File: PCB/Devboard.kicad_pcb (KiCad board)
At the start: 2 copper layers, 675 parts, among them CN1 APCI0120-P001A, J1 HR911105A_C12074, J10 I2C_7, J11 3.3V_I2C, J17 I2C_0, J2 USB3_B, J4 I2C_1, J5 I2C_2, J6 I2C_3, J7 I2C_4, J8 I2C_5, J9 I2C_6, Q1 IPB180P04P4L-02, Q2 IPB180P04P4L-02, SW1 SW_Push, U1 TVS2201DRBR, U10 TPS62822DLCR, U11 TPS62823DLCR, U12 TPS548A20RVER, U13 TPS7A4700RGWR, U14 TPS3700DSET, U15 TPS54824RNVR, U16 TPS54824RNVR, U17 TPS7A4700RGWR, U18 DW06, U19 TPS61088RHLR, U2 TPD6S300ARUKR, U20 TPS54824RNVR, U21 LM66100DCK, U22 TPS7A4700RGWR, U23 TPS7A4700RGWR, U24 TPS259470ARPWR, U25 TPS54824RNVR, U26 xczu4evfbvb900pkg, U27 RS3112-1.25XSF3, U28 MT25QU256ABA8ESF-0SIT TR, U29 FEMDNN032G-A3A55, U3 STUSB4500QTR, U30 TXS02612RTWR, U31 DP83867IRRGZR, U32 USB3320C-EZK-TR, U33 TPD4E05U06DQA, U34 CP2102N-A02-GQFN24, U35 TXB0108PW, U36 TCA9548APWR, U37 PCA9306, U39 TPD4E05U06DQA, U4 TPS2121RUXR, U40 USB2514B_Bi, U5 TPS259470ARPWR, U6 BQ25895RTWR, U7 BQ27441DRZR-G1A, U8 TPS62130RGTR, U9 XT60, Y1 25 MHz, Y2 25 MHz, Y4 26 MHz

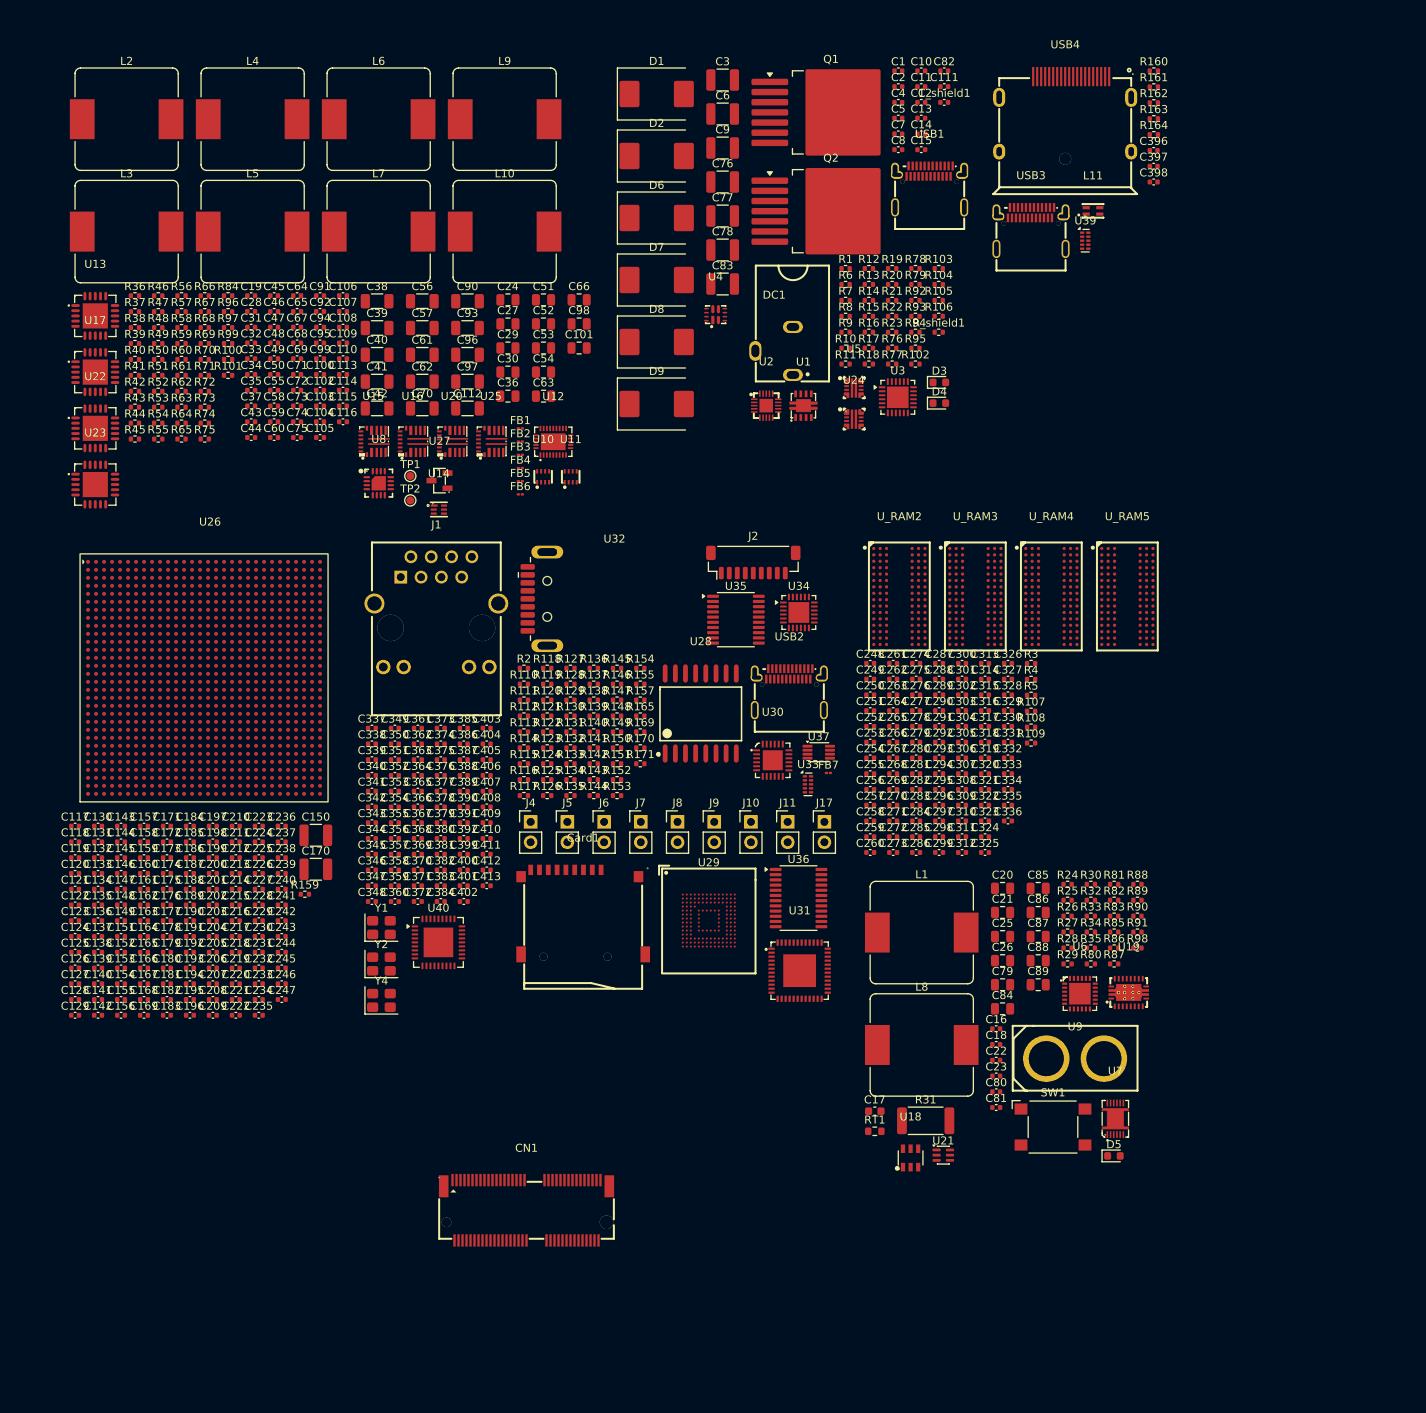
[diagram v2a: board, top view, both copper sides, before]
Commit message: Feat : Schematics Complete
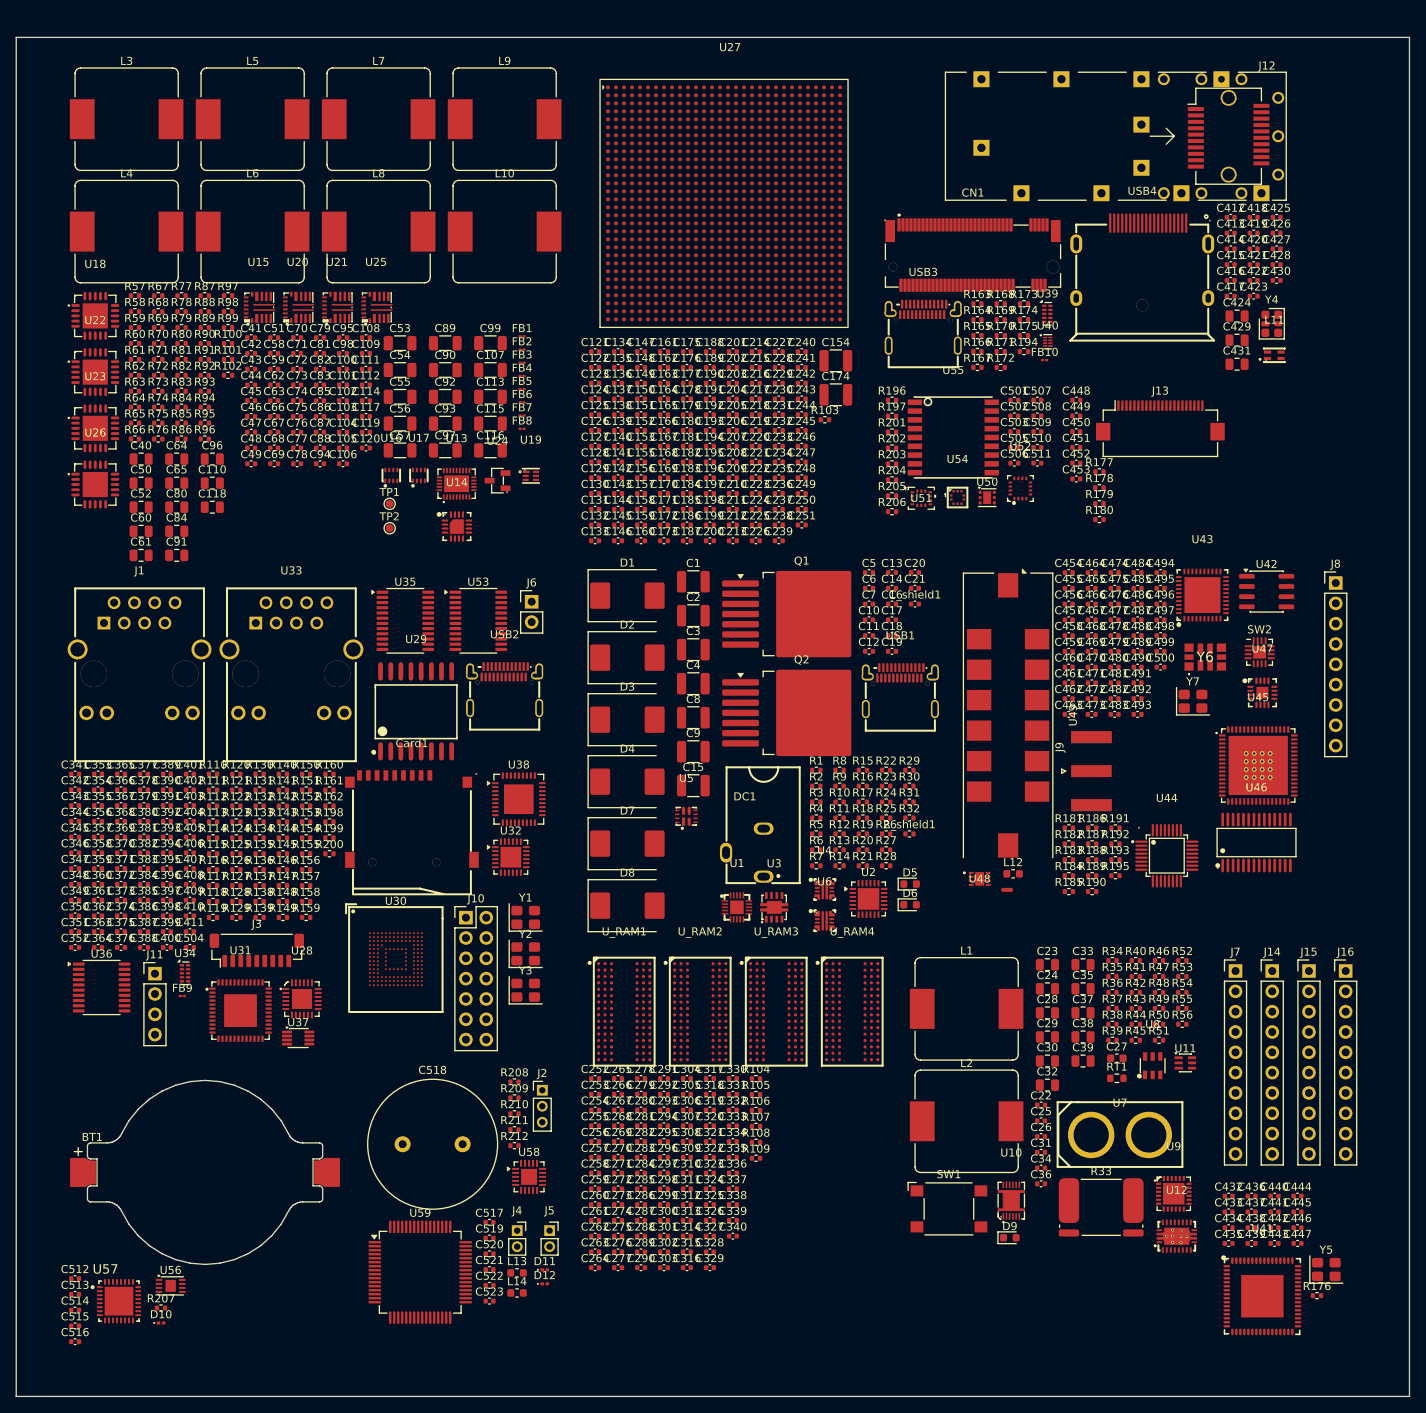
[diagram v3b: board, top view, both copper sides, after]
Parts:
- removed J17: I2C_0, Connector_PinHeader_2.54mm:PinHeader_1x02_P2.54mm_Vertical
- removed U_RAM5: MT40A512M16LY-075:E, Devboard_Footprints:FBGA-96_L13.5-W7.5-R16-C6-P0.80-TL
- added BT1: Battery_Cell, Battery:BatteryHolder_Keystone_1057_1x2032, F.Cu at (17.2, 138.2)
- added C393: 1uF, Capacitor_SMD:C_0402_1005Metric, F.Cu at (12.4, 96.3)
- added C394: 1uF, Capacitor_SMD:C_0402_1005Metric, F.Cu at (12.4, 98.2)
- added C395: 1uF, Capacitor_SMD:C_0402_1005Metric, F.Cu at (12.4, 100.2)
- added C414: 100nF, Capacitor_SMD:C_0402_1005Metric, F.Cu at (145.4, 22.7)
- added C415: 100nF, Capacitor_SMD:C_0402_1005Metric, F.Cu at (145.4, 24.7)
- added C416: 100nF, Capacitor_SMD:C_0402_1005Metric, F.Cu at (145.4, 26.7)
- added C417: 100nF, Capacitor_SMD:C_0402_1005Metric, F.Cu at (145.4, 28.6)
- added C418: 100nF, Capacitor_SMD:C_0402_1005Metric, F.Cu at (148.3, 18.8)
- added C419: 100nF, Capacitor_SMD:C_0402_1005Metric, F.Cu at (148.3, 20.8)
- added C420: 100nF, Capacitor_SMD:C_0402_1005Metric, F.Cu at (148.3, 22.7)
- added C421: 100nF, Capacitor_SMD:C_0402_1005Metric, F.Cu at (148.3, 24.7)
- added C422: 1nF, Capacitor_SMD:C_0402_1005Metric, F.Cu at (148.3, 26.7)
- added C423: 100nF, Capacitor_SMD:C_0402_1005Metric, F.Cu at (148.3, 28.6)
- added C424: 10uF, Capacitor_SMD:C_0805_2012Metric, F.Cu at (146.2, 31.1)
- added C425: 100nF, Capacitor_SMD:C_0402_1005Metric, F.Cu at (151.1, 18.8)
- added C426: 100nF, Capacitor_SMD:C_0402_1005Metric, F.Cu at (151.1, 20.8)
- added C427: 100nF, Capacitor_SMD:C_0402_1005Metric, F.Cu at (151.1, 22.7)
- added C428: 100nF, Capacitor_SMD:C_0402_1005Metric, F.Cu at (151.1, 24.7)
- added C429: 10uF, Capacitor_SMD:C_0805_2012Metric, F.Cu at (146.2, 34.1)
- added C430: 100nF, Capacitor_SMD:C_0402_1005Metric, F.Cu at (151.1, 26.7)
- added C431: 10uF, Capacitor_SMD:C_0805_2012Metric, F.Cu at (146.2, 37.2)
- added C432: 0.1uF, Capacitor_SMD:C_0402_1005Metric, F.Cu at (145.1, 141.1)
- added C433: 0.1uF, Capacitor_SMD:C_0402_1005Metric, F.Cu at (145.1, 143.1)
- added C434: 0.1uF, Capacitor_SMD:C_0402_1005Metric, F.Cu at (145.1, 145.1)
- added C435: 0.1uF, Capacitor_SMD:C_0402_1005Metric, F.Cu at (145.1, 147.1)
- added C436: 0.1uF, Capacitor_SMD:C_0402_1005Metric, F.Cu at (148.0, 141.1)
- added C437: 0.1uF, Capacitor_SMD:C_0402_1005Metric, F.Cu at (148.0, 143.1)
- added C438: 0.1uF, Capacitor_SMD:C_0402_1005Metric, F.Cu at (148.0, 145.1)
- added C439: 0.1uF, Capacitor_SMD:C_0402_1005Metric, F.Cu at (148.0, 147.1)
- added C440: 0.1uF, Capacitor_SMD:C_0402_1005Metric, F.Cu at (150.9, 141.1)
- added C441: 0.1uF, Capacitor_SMD:C_0402_1005Metric, F.Cu at (150.9, 143.1)
- added C442: 0.1uF, Capacitor_SMD:C_0402_1005Metric, F.Cu at (150.9, 145.1)
- added C443: 0.1uF, Capacitor_SMD:C_0402_1005Metric, F.Cu at (150.9, 147.1)
- added C444: 0.1uF, Capacitor_SMD:C_0402_1005Metric, F.Cu at (153.7, 141.1)
- added C445: 0.1uF, Capacitor_SMD:C_0402_1005Metric, F.Cu at (153.7, 143.1)
- added C446: 0.1uF, Capacitor_SMD:C_0402_1005Metric, F.Cu at (153.7, 145.1)
- added C447: 0.1uF, Capacitor_SMD:C_0402_1005Metric, F.Cu at (153.7, 147.1)
- added C448: 100nF, Capacitor_SMD:C_0402_1005Metric, F.Cu at (126.1, 41.6)
- added C449: 100nF, Capacitor_SMD:C_0402_1005Metric, F.Cu at (126.1, 43.6)
- added C450: 100nF, Capacitor_SMD:C_0402_1005Metric, F.Cu at (126.1, 45.6)
- added C451: 10uF, Capacitor_SMD:C_0402_1005Metric, F.Cu at (126.1, 47.6)
- added C452: 100nF, Capacitor_SMD:C_0402_1005Metric, F.Cu at (126.1, 49.5)
- added C453: 10uF, Capacitor_SMD:C_0402_1005Metric, F.Cu at (126.1, 51.5)
- added C454: 10uF, Capacitor_SMD:C_0402_1005Metric, F.Cu at (125.1, 63.2)
- added C455: 10uF, Capacitor_SMD:C_0402_1005Metric, F.Cu at (125.1, 65.2)
- added C456: 100nF, Capacitor_SMD:C_0402_1005Metric, F.Cu at (125.1, 67.1)
- added C457: 1uF, Capacitor_SMD:C_0402_1005Metric, F.Cu at (125.1, 69.1)
- added C458: 100nF, Capacitor_SMD:C_0402_1005Metric, F.Cu at (125.1, 71.1)
- added C459: 1uF, Capacitor_SMD:C_0402_1005Metric, F.Cu at (125.1, 73.0)
- added C460: 100nF, Capacitor_SMD:C_0402_1005Metric, F.Cu at (125.1, 75.0)
- added C461: 100nF, Capacitor_SMD:C_0402_1005Metric, F.Cu at (125.1, 77.0)
- added C462: 100nF, Capacitor_SMD:C_0402_1005Metric, F.Cu at (125.1, 79.0)
- added C463: 100nF, Capacitor_SMD:C_0402_1005Metric, F.Cu at (125.1, 80.9)
- added C464: 100nF, Capacitor_SMD:C_0402_1005Metric, F.Cu at (128.0, 63.2)
- added C465: 10uF, Capacitor_SMD:C_0402_1005Metric, F.Cu at (128.0, 65.2)
- added C466: 1uF, Capacitor_SMD:C_0402_1005Metric, F.Cu at (128.0, 67.1)
- added C467: 100nF, Capacitor_SMD:C_0402_1005Metric, F.Cu at (128.0, 69.1)
- added C468: 1uF, Capacitor_SMD:C_0402_1005Metric, F.Cu at (128.0, 71.1)
- added C469: 10uF, Capacitor_SMD:C_0402_1005Metric, F.Cu at (128.0, 73.0)
- added C470: 1uF, Capacitor_SMD:C_0402_1005Metric, F.Cu at (128.0, 75.0)
- added C471: 100nF, Capacitor_SMD:C_0402_1005Metric, F.Cu at (128.0, 77.0)
- added C472: 1uF, Capacitor_SMD:C_0402_1005Metric, F.Cu at (128.0, 79.0)
- added C473: 0.56 nF, Capacitor_SMD:C_0402_1005Metric, F.Cu at (128.0, 80.9)
- added C474: 330 nF, Capacitor_SMD:C_0402_1005Metric, F.Cu at (130.9, 63.2)
- added C475: 3.3 nF, Capacitor_SMD:C_0402_1005Metric, F.Cu at (130.9, 65.2)
- added C476: 100nF, Capacitor_SMD:C_0402_1005Metric, F.Cu at (130.9, 67.1)
- added C477: 100pF, Capacitor_SMD:C_0402_1005Metric, F.Cu at (130.9, 69.1)
- added C478: 100pF, Capacitor_SMD:C_0402_1005Metric, F.Cu at (130.9, 71.1)
- added C479: 1uF, Capacitor_SMD:C_0402_1005Metric, F.Cu at (130.9, 73.0)
- added C480: 100nF, Capacitor_SMD:C_0402_1005Metric, F.Cu at (130.9, 75.0)
- added C481: 22pF, Capacitor_SMD:C_0402_1005Metric, F.Cu at (130.9, 77.0)
- added C482: 22pF, Capacitor_SMD:C_0402_1005Metric, F.Cu at (130.9, 79.0)
- added C483: 0.1uF, Capacitor_SMD:C_0402_1005Metric, F.Cu at (130.9, 80.9)
- added C484: 10uF, Capacitor_SMD:C_0402_1005Metric, F.Cu at (133.7, 63.2)
- added C485: 0.1uF, Capacitor_SMD:C_0402_1005Metric, F.Cu at (133.7, 65.2)
- added C486: 10uF, Capacitor_SMD:C_0402_1005Metric, F.Cu at (133.7, 67.1)
- added C487: 0.1uF, Capacitor_SMD:C_0402_1005Metric, F.Cu at (133.7, 69.1)
- added C488: 10uF, Capacitor_SMD:C_0402_1005Metric, F.Cu at (133.7, 71.1)
- added C489: 0.1uF, Capacitor_SMD:C_0402_1005Metric, F.Cu at (133.7, 73.0)
- added C490: 10uF, Capacitor_SMD:C_0402_1005Metric, F.Cu at (133.7, 75.0)
- added C491: 100nF, Capacitor_SMD:C_0402_1005Metric, F.Cu at (133.7, 77.0)
- added C492: 100nF, Capacitor_SMD:C_0402_1005Metric, F.Cu at (133.7, 79.0)
- added C493: 0.1uF, Capacitor_SMD:C_0402_1005Metric, F.Cu at (133.7, 80.9)
- added C494: 0.1uF, Capacitor_SMD:C_0402_1005Metric, F.Cu at (136.6, 63.2)
- added C495: 100pF, Capacitor_SMD:C_0402_1005Metric, F.Cu at (136.6, 65.2)
- added C496: 100pF, Capacitor_SMD:C_0402_1005Metric, F.Cu at (136.6, 67.1)
- added C497: 1uF, Capacitor_SMD:C_0402_1005Metric, F.Cu at (136.6, 69.1)
- added C498: 1uF, Capacitor_SMD:C_0402_1005Metric, F.Cu at (136.6, 71.1)
- added C499: 0.1 uF, Capacitor_SMD:C_0402_1005Metric, F.Cu at (136.6, 73.0)
- added C500: 100nF, Capacitor_SMD:C_0402_1005Metric, F.Cu at (136.6, 75.0)
- added C501: 0.1uF, Capacitor_SMD:C_0402_1005Metric, F.Cu at (118.3, 41.6)
- added C502: 0.1uF, Capacitor_SMD:C_0402_1005Metric, F.Cu at (118.3, 43.6)
- added C503: 0.1uF, Capacitor_SMD:C_0402_1005Metric, F.Cu at (118.3, 45.6)
- added C504: 0.1uF, Capacitor_SMD:C_0402_1005Metric, F.Cu at (15.3, 110.1)
- added C505: 0.1uF, Capacitor_SMD:C_0402_1005Metric, F.Cu at (118.3, 47.6)
- added C506: 0.1uF, Capacitor_SMD:C_0402_1005Metric, F.Cu at (118.3, 49.5)
- added C507: 10uF, Capacitor_SMD:C_0402_1005Metric, F.Cu at (121.2, 41.6)
- added C508: 0.1uF, Capacitor_SMD:C_0402_1005Metric, F.Cu at (121.2, 43.6)
- added C509: 0.1uF, Capacitor_SMD:C_0402_1005Metric, F.Cu at (121.2, 45.6)
- added C510: 0.1uF, Capacitor_SMD:C_0402_1005Metric, F.Cu at (121.2, 47.6)
- added C511: 0.1uF, Capacitor_SMD:C_0402_1005Metric, F.Cu at (121.2, 49.5)
- added C512: 0.1uF, Capacitor_SMD:C_0402_1005Metric, F.Cu at (0.94, 151.5)
- added C513: 0.1uF, Capacitor_SMD:C_0402_1005Metric, F.Cu at (0.94, 153.4)
- added C514: 0.1uF, Capacitor_SMD:C_0402_1005Metric, F.Cu at (0.94, 155.4)
- added C515: 0.1uF, Capacitor_SMD:C_0402_1005Metric, F.Cu at (0.94, 157.4)
- added C516: 0.1uF, Capacitor_SMD:C_0402_1005Metric, F.Cu at (0.94, 159.3)
- added C517: 0.1uF, Capacitor_SMD:C_0402_1005Metric, F.Cu at (52.7, 144.4)
- added C518: 22F 5.5V, Capacitor_THT:C_Radial_D16.0mm_H31.5mm_P7.50mm, F.Cu at (41.9, 134.7)
- added C519: 0.1uF, Capacitor_SMD:C_0402_1005Metric, F.Cu at (52.7, 146.4)
- added C520: 0.1uF, Capacitor_SMD:C_0402_1005Metric, F.Cu at (52.7, 148.4)
- added C521: 0.1uF, Capacitor_SMD:C_0402_1005Metric, F.Cu at (52.7, 150.3)
- added C522: 0.1uF, Capacitor_SMD:C_0402_1005Metric, F.Cu at (52.7, 152.3)
- added C523: 0.1uF, Capacitor_SMD:C_0402_1005Metric, F.Cu at (52.7, 154.3)
- added D10: RB521S30, Diode_SMD:D_0201_0603Metric, F.Cu at (11.7, 157.0)
- added D11: RB521S30, Diode_SMD:D_0201_0603Metric, F.Cu at (59.6, 150.4)
- added D12: RB521S30, Diode_SMD:D_0201_0603Metric, F.Cu at (59.6, 152.1)
- added FB10: 120Ω@100MHz, Inductor_SMD:L_01005_0402Metric, F.Cu at (122.1, 36.6)
- added FB8: 120Ω@100MHz, Inductor_SMD:L_01005_0402Metric, F.Cu at (56.8, 45.2)
- added FB9: BLM18, Inductor_SMD:L_01005_0402Metric, F.Cu at (14.3, 116.1)
- added J12: SFP+, Connector:Connector_SFP_and_Cage, F.Cu at (151.3, 8.65)
- added J13: Conn_01x22, Connector_FFC-FPC:Hirose_FH12-22S-0.5SH_1x22-1MP_P0.50mm_Horizontal, F.Cu at (136.6, 44.2)
- added J14: Conn_01x10, Connector_PinHeader_2.54mm:PinHeader_1x10_P2.54mm_Vertical, F.Cu at (150.6, 113.0)
- added J15: Conn_01x10, Connector_PinHeader_2.54mm:PinHeader_1x10_P2.54mm_Vertical, F.Cu at (155.2, 113.0)
- added J16: Conn_01x10, Connector_PinHeader_2.54mm:PinHeader_1x10_P2.54mm_Vertical, F.Cu at (159.8, 113.0)
- added J3: USB3_B, Connector_JST:JST_SH_BM09B-SRSS-TB_1x09-1MP_P1.00mm_Vertical, F.Cu at (23.6, 110.4)
- added L12: 220 nH, Inductor_SMD:L_0603_1608Metric, F.Cu at (118.2, 100.9)
- added L13: 220 nH, Inductor_SMD:L_0603_1608Metric, F.Cu at (56.2, 150.7)
- added L14: 220 nH, Inductor_SMD:L_0603_1608Metric, F.Cu at (56.2, 153.2)
- added NT1: NetTie_2, NetTie:NetTie-2_SMD_Pad0.5mm, F.Cu at (117.4, 102.9)
- added R156: 2.2kΩ, Resistor_SMD:R_0402_1005Metric, F.Cu at (29.8, 100.3)
- added R158: 10kΩ, Resistor_SMD:R_0402_1005Metric, F.Cu at (29.8, 104.3)
- added R166: 100kΩ, Resistor_SMD:R_0402_1005Metric, F.Cu at (113.7, 35.6)
- added R167: 1MΩ, Resistor_SMD:R_0402_1005Metric, F.Cu at (113.7, 37.6)
- added R168: 50Ω, Resistor_SMD:R_0402_1005Metric, F.Cu at (116.6, 29.6)
- added R172: 10kΩ, Resistor_SMD:R_0402_1005Metric, F.Cu at (116.6, 37.6)
- added R173: 10kΩ, Resistor_SMD:R_0402_1005Metric, F.Cu at (119.5, 29.6)
- added R174: 10kΩ, Resistor_SMD:R_0402_1005Metric, F.Cu at (119.5, 31.6)
- added R175: 50Ω, Resistor_SMD:R_0402_1005Metric, F.Cu at (119.5, 33.6)
- added R176: 1MΩ, Resistor_SMD:R_0402_1005Metric, F.Cu at (156.2, 153.6)
- added R177: 4.7kΩ, Resistor_SMD:R_0402_1005Metric, F.Cu at (129.0, 50.6)
- added R178: 4.7kΩ, Resistor_SMD:R_0402_1005Metric, F.Cu at (129.0, 52.6)
- added R179: 10kΩ, Resistor_SMD:R_0402_1005Metric, F.Cu at (129.0, 54.6)
- added R180: 10kΩ, Resistor_SMD:R_0402_1005Metric, F.Cu at (129.0, 56.6)
- added R181: 4.7kΩ, Resistor_SMD:R_0402_1005Metric, F.Cu at (125.2, 95.1)
- added R182: 27Ω, Resistor_SMD:R_0402_1005Metric, F.Cu at (125.2, 97.1)
- added R183: 10Ω, Resistor_SMD:R_0402_1005Metric, F.Cu at (125.2, 99.1)
- added R184: 27Ω, Resistor_SMD:R_0402_1005Metric, F.Cu at (125.2, 101.1)
- added R185: 27Ω, Resistor_SMD:R_0402_1005Metric, F.Cu at (125.2, 103.1)
- added R186: 50Ω, Resistor_SMD:R_0402_1005Metric, F.Cu at (128.1, 95.1)
- added R187: 10Ω, Resistor_SMD:R_0402_1005Metric, F.Cu at (128.1, 97.1)
- added R188: 10kΩ, Resistor_SMD:R_0402_1005Metric, F.Cu at (128.1, 99.1)
- added R189: 10kΩ, Resistor_SMD:R_0402_1005Metric, F.Cu at (128.1, 101.1)
- added R190: 10kΩ, Resistor_SMD:R_0402_1005Metric, F.Cu at (128.1, 103.1)
- added R191: 1.92kΩ, Resistor_SMD:R_0402_1005Metric, F.Cu at (131.0, 95.1)
- added R192: 50Ω, Resistor_SMD:R_0402_1005Metric, F.Cu at (131.0, 97.1)
- added R193: 50Ω, Resistor_SMD:R_0402_1005Metric, F.Cu at (131.0, 99.1)
- added R194: 10kΩ, Resistor_SMD:R_0402_1005Metric, F.Cu at (119.5, 35.6)
- added R195: 50Ω, Resistor_SMD:R_0402_1005Metric, F.Cu at (131.0, 101.1)
- added R196: 5kΩ, Resistor_SMD:R_0402_1005Metric, F.Cu at (103.1, 41.7)
- added R197: 5kΩ, Resistor_SMD:R_0402_1005Metric, F.Cu at (103.1, 43.6)
- added R198: 10kΩ, Resistor_SMD:R_0402_1005Metric, F.Cu at (32.7, 94.4)
- added R199: 2.2kΩ, Resistor_SMD:R_0402_1005Metric, F.Cu at (32.7, 96.4)
- added R200: 2.2kΩ, Resistor_SMD:R_0402_1005Metric, F.Cu at (32.7, 98.3)
- added R201: 5kΩ, Resistor_SMD:R_0402_1005Metric, F.Cu at (103.1, 45.6)
- added R202: 5kΩ, Resistor_SMD:R_0402_1005Metric, F.Cu at (103.1, 47.6)
- added R203: 5kΩ, Resistor_SMD:R_0402_1005Metric, F.Cu at (103.1, 49.6)
- added R204: 5kΩ, Resistor_SMD:R_0402_1005Metric, F.Cu at (103.1, 51.6)
- added R205: 5kΩ, Resistor_SMD:R_0402_1005Metric, F.Cu at (103.1, 53.6)
- added R206: 5kΩ, Resistor_SMD:R_0402_1005Metric, F.Cu at (103.1, 55.6)
- added R207: 10kΩ, Resistor_SMD:R_0402_1005Metric, F.Cu at (11.7, 155.1)
- added R208: 4.02MΩ, Resistor_SMD:R_0402_1005Metric, F.Cu at (55.9, 126.9)
- added R209: 1MΩ, Resistor_SMD:R_0402_1005Metric, F.Cu at (55.9, 128.9)
- added R210: 1MΩ, Resistor_SMD:R_0402_1005Metric, F.Cu at (55.9, 130.9)
- added R211: 3MΩ, Resistor_SMD:R_0402_1005Metric, F.Cu at (55.9, 132.8)
- added R212: 10kΩ, Resistor_SMD:R_0402_1005Metric, F.Cu at (55.9, 134.8)
- added SW2: SW_SPDT, Devboard_Footprints:LFCSP-16-1EP_3x3mm_P0.5mm_EP1.6x1.6mm, F.Cu at (149.0, 73.2)
- added U38: USB2514B_Bi, Package_DFN_QFN:QFN-36-1EP_6x6mm_P0.5mm_EP3.7x3.7mm, F.Cu at (56.4, 91.5)
- added U41: SI5341A-D12636-GM, Devboard_Footprints:QFN-64_L9.0-W9.0-P0.50-TL-EP5.2, F.Cu at (149.3, 153.7)
- added U42: REF5025AD, Package_SO:SOIC-8_3.9x4.9mm_P1.27mm, F.Cu at (149.9, 65.6)
- added U43: LMX2594RHAR, Devboard_Footprints:QFN-40_L6.0-W6.0-P0.50-BL-EP4.5, F.Cu at (141.8, 66.0)
- added U44: ADS131M08IPBS, Devboard_Footprints:TQFP-32_L5.0-W5.0-P0.50-LS7.0-TL, F.Cu at (137.4, 98.6)
- added U45: ADS4245IRGCT, Devboard_Footprints:VQFN-64_L9.0-W9.0-P0.50-TL-EP7.4, F.Cu at (148.8, 87.3)
- added U46: AD9744ARUZRL7, Devboard_Footprints:TSSOP-28_L9.7-W4.4-P0.65-LS6.4-BL, F.Cu at (148.6, 96.9)
- added U47: THS4509RGTT, Devboard_Footprints:VQFN-16_L3.0-W3.0-P0.50-TL-EP1.5, F.Cu at (149.3, 78.2)
- added U48: ADL8100ACPZN, Devboard_Footprints:CP-8-30_ADI, F.Cu at (114.0, 101.5)
- added U49: BPF-A355, RF_Mini-Circuits:Mini-Circuits_HQ1157, F.Cu at (117.6, 81.0)
- added U50: TMP117DRVR, Package_SON:WSON-6-1EP_2x2mm_P0.65mm_EP1x1.6mm, F.Cu at (114.9, 53.8)
- added U51: ICM-42688-P, Custom_Footprints:LGA14_2P5X3X0P91_TDK-L, F.Cu at (106.7, 53.9)
- added U52: MMC5983MA, Devboard_Footprints:LGA-16_L3.0-W3.0-P0.50-BL_SQ, F.Cu at (119.1, 52.7)
- added U53: TCA9548APWR, Package_SO:TSSOP-24_4.4x7.8mm_P0.65mm, F.Cu at (51.3, 69.2)
- added U54: BMP581, Devboard_Footprints:LGA-10_L2.0-W2.0-P0.50-TL_BMP581, F.Cu at (111.2, 53.8)
- added U55: MAX-M10S-00B, Devboard_Footprints:SMD-18_L10.1-W9.7-P1.10-TL_SKG09F, F.Cu at (110.7, 46.3)
- added U56: ATECC608B-MAHDA, Package_DFN_QFN:DFN-8-1EP_3x2mm_P0.5mm_EP1.3x1.5mm, F.Cu at (12.9, 152.4)
- added U57: OPTIGA TPM SLB 9673 FW26, Devboard_Footprints:QFN50P500X500X60-33N-V2, F.Cu at (6.42, 154.3)
- added U58: BQ25570, Package_DFN_QFN:QFN-20-1EP_3.5x3.5mm_P0.5mm_EP2x2mm, F.Cu at (57.7, 138.7)
- added U59: STM32G0B1RBT6, Package_QFP:LQFP-64_10x10mm_P0.5mm, F.Cu at (44.1, 150.7)
- added U_RAM1: MT40A512M16LY-075:E, Devboard_Footprints:FBGA-96_L13.5-W7.5-R16-C6-P0.80-TL, F.Cu at (69.6, 118.1)
- added Y3: 26 MHz, Crystal:Crystal_SMD_3225-4Pin_3.2x2.5mm, F.Cu at (57.3, 115.4)
- added Y5: ECS_480-8-37-A-D-P-TR, Crystal:Crystal_SMD_3225-4Pin_3.2x2.5mm, F.Cu at (157.3, 150.3)
- added Y6: SiT5356AI-FP-25VT-16.367667, Devboard_Footprints:Ceramic_QFN_5032_10pins, F.Cu at (142.2, 73.8)
- added Y7: 25 MHz, Crystal:Crystal_SMD_3225-4Pin_3.2x2.5mm, F.Cu at (140.7, 79.3)
- C1: value 1uF 25V -> 1uF; footprint Capacitor_SMD:C_0402_1005Metric -> Capacitor_SMD:C_1210_3225Metric
- C10: value 2.2nF 25V -> 1uF 25V
- C100: value 10nF -> 10uF
- C101: value 22uf 25v -> 1uF; footprint Capacitor_SMD:C_0805_2012Metric -> Capacitor_SMD:C_0402_1005Metric
- C102, C45: value 4.7nF 50V -> 1uF
- C104: value 22pF -> 0.1uF 25v
- C107, C113: value 0.1uF 25V -> 47uF; footprint Capacitor_SMD:C_0402_1005Metric -> Capacitor_SMD:C_1206_3216Metric
- C109: value 0.1uF 25V -> 10nF
- C11: value 0.1uF 25V -> 0.1uF 50V X7R
- C110, C91: value 10uF -> 22uf 25v; footprint Capacitor_SMD:C_0402_1005Metric -> Capacitor_SMD:C_0805_2012Metric
- C111, C14: value 10nF 25V -> 4.7nF 50V
- C112: value 47uF -> 100pF; footprint Capacitor_SMD:C_1206_3216Metric -> Capacitor_SMD:C_0402_1005Metric
- C114: value 10uF -> 22pF
- C115: value 0.1uF 25V -> 47uF 6.3V; footprint Capacitor_SMD:C_0402_1005Metric -> Capacitor_SMD:C_1206_3216Metric
- C116: value 10uF -> 47uF 6.3V; footprint Capacitor_SMD:C_0402_1005Metric -> Capacitor_SMD:C_1206_3216Metric
- C117, C342, C344, C346, C350, C357, C359, C361, C391: value 0.1uF -> 1uF
- C118: value 0.1uF -> 22uf 25v; footprint Capacitor_SMD:C_0402_1005Metric -> Capacitor_SMD:C_0805_2012Metric
- C119: value 0.1uF -> 0.1uF 25V
- C12: value 0.1uF 25V -> 10nF 25V
- C120: value 0.1uF -> 10uF
- C13: value 0.1uF 50V -> 10nF 25V
- C15: value 0.1uF 50V -> 100uF 35V; footprint Capacitor_SMD:C_0402_1005Metric -> Capacitor_SMD:C_1210_3225Metric
- C150, C170: value 47uF -> 0.1uF; footprint Capacitor_SMD:C_1210_3225Metric -> Capacitor_SMD:C_0402_1005Metric
- C154, C174: value 0.1uF -> 47uF; footprint Capacitor_SMD:C_0402_1005Metric -> Capacitor_SMD:C_1210_3225Metric
- C16: value 47nF -> 2.2nF 25V
- C17: value 4.7uF -> 0.1uF 25V; footprint Capacitor_SMD:C_0603_1608Metric -> Capacitor_SMD:C_0402_1005Metric
- C18, C72: value 1uF -> 0.1uF 25V
- C19: value 10uF -> 0.1uF 50V
- C2: value 1uF 25V -> 100uF 35V; footprint Capacitor_SMD:C_0402_1005Metric -> Capacitor_SMD:C_1210_3225Metric
- C20: value 22uF -> 10nF 25V; footprint Capacitor_SMD:C_0805_2012Metric -> Capacitor_SMD:C_0402_1005Metric
- C21: value 22uF -> 0.1uF 50V; footprint Capacitor_SMD:C_0805_2012Metric -> Capacitor_SMD:C_0402_1005Metric
- C22: value 10uF -> 47nF
- C23: value 0.47uF -> 22uF; footprint Capacitor_SMD:C_0402_1005Metric -> Capacitor_SMD:C_0805_2012Metric
- C25: value 22uF -> 1uF; footprint Capacitor_SMD:C_0805_2012Metric -> Capacitor_SMD:C_0402_1005Metric
- C26: value 22uF -> 100nF; footprint Capacitor_SMD:C_0805_2012Metric -> Capacitor_SMD:C_0402_1005Metric
- C27: value 22uF -> 4.7uF; footprint Capacitor_SMD:C_0805_2012Metric -> Capacitor_SMD:C_0603_1608Metric
- C28: value 10uF -> 22uF; footprint Capacitor_SMD:C_0402_1005Metric -> Capacitor_SMD:C_0805_2012Metric
- C3: value 100uF 35V -> 1uF
- C31: value 0.1uF, 25V -> 100nF
- C32: value 10nF, 10V -> 1uF; footprint Capacitor_SMD:C_0402_1005Metric -> Capacitor_SMD:C_0805_2012Metric
- C33: value 10nF -> 1uF; footprint Capacitor_SMD:C_0402_1005Metric -> Capacitor_SMD:C_0805_2012Metric
- C339, C341, C343, C345, C349, C356, C360, C387, C399, C401, C402, C403, C411: value 1uF -> 0.1uF
- C34: value 100pF -> 0.47uF
- C35: value 3.3nF -> 10nF; footprint Capacitor_SMD:C_0402_1005Metric -> Capacitor_SMD:C_0805_2012Metric
- C36: value 22uF, 6.3V -> 10uF; footprint Capacitor_SMD:C_0805_2012Metric -> Capacitor_SMD:C_0402_1005Metric
- C364, C365, C366, C374: value 1nF -> 0.1uF
- C369, C381, C382, C383, C392: value 0.1uF -> 1nF
- C37: value 10uF -> 1uF; footprint Capacitor_SMD:C_0402_1005Metric -> Capacitor_SMD:C_0805_2012Metric
- C372: value 1nF -> 33pF
- C373, C408, C409: value 0.1uF -> 33pF
- C376: value 22uF -> 0.1uF
- C379, C405, C406: value 33pF -> 0.1uF
- C38: value 47uF -> 0.1uF; footprint Capacitor_SMD:C_1206_3216Metric -> Capacitor_SMD:C_0805_2012Metric
- C380: value 33pF -> 1nF
- C385: value 0.1uF -> 22uF
- C39: value 47uF,4V -> 10nF; footprint Capacitor_SMD:C_1206_3216Metric -> Capacitor_SMD:C_0805_2012Metric
- C396: value 100nF -> 1uF
- C397: value 100nF -> 0.1uF
- C398: value 1nF -> 1uF
- C4: value 0.1uF 50V X7R -> 100nF; footprint Capacitor_SMD:C_0402_1005Metric -> Capacitor_SMD:C_1210_3225Metric
- C40: value 47uF,4V -> 22uF, 6.3V; footprint Capacitor_SMD:C_1206_3216Metric -> Capacitor_SMD:C_0805_2012Metric
- C41: value 47uF,4V -> 0.1uF, 25V; footprint Capacitor_SMD:C_1206_3216Metric -> Capacitor_SMD:C_0402_1005Metric
- C412: value 0.1uF -> 100nF
- C413: value 1nF -> 100nF
- C42: value 47uF,4V -> 100pF; footprint Capacitor_SMD:C_1206_3216Metric -> Capacitor_SMD:C_0402_1005Metric
- C43: value 0.1uF, 25V -> 100pF
- C44: value 1uF -> 10nF, 10V
- C46: value 100pF -> 10nF
- C47: value 2.2nF -> 3.3nF
- C49: value 1uF -> 0.1uF, 25V
- C5: value 2.2uF -> 1uF 25V
- C50: value 0.1uF -> 22uF; footprint Capacitor_SMD:C_0402_1005Metric -> Capacitor_SMD:C_0805_2012Metric
- C51: value 22uF -> 2.2nF; footprint Capacitor_SMD:C_0805_2012Metric -> Capacitor_SMD:C_0402_1005Metric
- C53, C54: value 22uf 25v -> 47uF,4V; footprint Capacitor_SMD:C_0805_2012Metric -> Capacitor_SMD:C_1206_3216Metric
- C55: value 0.1uF 25v -> 47uF,4V; footprint Capacitor_SMD:C_0402_1005Metric -> Capacitor_SMD:C_1206_3216Metric
- C56: value 47uF 6.3V -> 47uF,4V
- C57, C97: value 47uF 6.3V -> 47uF
- C58, C69: value 22pF -> 10uF
- C59, C73: value 100pF -> 10uF
- C6: value 100uF 35V -> 2.2uF; footprint Capacitor_SMD:C_1210_3225Metric -> Capacitor_SMD:C_0402_1005Metric
- C60, C65: value 10nF -> 22uF; footprint Capacitor_SMD:C_0402_1005Metric -> Capacitor_SMD:C_0805_2012Metric
- C61: value 47uF 6.3V -> 22uF; footprint Capacitor_SMD:C_1206_3216Metric -> Capacitor_SMD:C_0805_2012Metric
- C62: value 47uF 6.3V -> 1uF; footprint Capacitor_SMD:C_1206_3216Metric -> Capacitor_SMD:C_0402_1005Metric
- C63, C98: value 22uf 25v -> 10uF; footprint Capacitor_SMD:C_0805_2012Metric -> Capacitor_SMD:C_0402_1005Metric
- C64: value 0.1uF 25v -> 22uF; footprint Capacitor_SMD:C_0402_1005Metric -> Capacitor_SMD:C_0805_2012Metric
- C66: value 22uf 25v -> 0.1uF 25V; footprint Capacitor_SMD:C_0805_2012Metric -> Capacitor_SMD:C_0402_1005Metric
- C67: value 4.7nF 50V -> 10uF
- C68: value 100pF -> 0.1uF 25V
- C7: value 10nF 25V -> 100nF
- C70: value 47uF -> 0.1uF 25V; footprint Capacitor_SMD:C_1206_3216Metric -> Capacitor_SMD:C_0402_1005Metric
- C74, C94: value 10uF -> 0.1uF 25V
- C75: value 0.1uF 25V -> 10uF
- C76: value 1uF -> 0.1uF 25v; footprint Capacitor_SMD:C_1210_3225Metric -> Capacitor_SMD:C_0402_1005Metric
- C77: value 1uF -> 0.1uF; footprint Capacitor_SMD:C_1210_3225Metric -> Capacitor_SMD:C_0402_1005Metric
- C78: value 100nF -> 0.1uF 25v; footprint Capacitor_SMD:C_1210_3225Metric -> Capacitor_SMD:C_0402_1005Metric
- C79: value 22uF -> 10nF; footprint Capacitor_SMD:C_0805_2012Metric -> Capacitor_SMD:C_0402_1005Metric
- C8: value 4.7nF 50V -> 1uF; footprint Capacitor_SMD:C_0402_1005Metric -> Capacitor_SMD:C_1210_3225Metric
- C80: value 100nF -> 22uf 25v; footprint Capacitor_SMD:C_0402_1005Metric -> Capacitor_SMD:C_0805_2012Metric
- C81: value 100nF -> 4.7nF 50V
- C82: value 100nF -> 100pF
- C83: value 1uF -> 10nF; footprint Capacitor_SMD:C_1210_3225Metric -> Capacitor_SMD:C_0402_1005Metric
- C84: value 1uF -> 22uf 25v
- C85: value 0.1uF -> 4.7nF 50V; footprint Capacitor_SMD:C_0805_2012Metric -> Capacitor_SMD:C_0402_1005Metric
- C86: value 10nF -> 100pF; footprint Capacitor_SMD:C_0805_2012Metric -> Capacitor_SMD:C_0402_1005Metric
- C87: value 10nF -> 22pF; footprint Capacitor_SMD:C_0805_2012Metric -> Capacitor_SMD:C_0402_1005Metric
- C88: value 1uF -> 22pF; footprint Capacitor_SMD:C_0805_2012Metric -> Capacitor_SMD:C_0402_1005Metric
- C89: value 1uF -> 47uF 6.3V; footprint Capacitor_SMD:C_0805_2012Metric -> Capacitor_SMD:C_1206_3216Metric
- C90, C93: value 47uF -> 47uF 6.3V
- C92: value 1uF -> 47uF 6.3V; footprint Capacitor_SMD:C_0402_1005Metric -> Capacitor_SMD:C_1206_3216Metric
- C95: value 1uF -> 10uF
- C96: value 47uF 6.3V -> 22uf 25v; footprint Capacitor_SMD:C_1206_3216Metric -> Capacitor_SMD:C_0805_2012Metric
- C99: value 0.1uF 25v -> 47uF; footprint Capacitor_SMD:C_0402_1005Metric -> Capacitor_SMD:C_1206_3216Metric
- CN1: value APCI0120-P001A -> 1-2199230-6; footprint Devboard_Footprints:CONN-SMD_APCI0120-P001A -> Devboard_Footprints:PCIE-SMD_1-2199230-6
- D1: value 15V -> SMBJ20A
- D2: value TP7.OSMD24CA-XC -> 15V
- D3: value Red -> TP7.OSMD24CA-XC; footprint LED_SMD:LED_0603_1608Metric -> Diode_SMD:D_SMC
- D4: value Green -> LSMB24CAH; footprint LED_SMD:LED_0603_1608Metric -> Diode_SMD:D_SMC
- D5: value Green -> Red
- D6: value LSMB24CAH -> Green; footprint Diode_SMD:D_SMC -> LED_SMD:LED_0603_1608Metric
- D7: value SMBJ20A -> D_Schottky
- D9: value D_Schottky -> Green; footprint Diode_SMD:D_SMC -> LED_SMD:LED_0603_1608Metric
- FB7: value BLM18 -> 120Ω@100MHz
- J10: value I2C_7 -> Conn_02x07_Odd_Even; footprint Connector_PinHeader_2.54mm:PinHeader_1x02_P2.54mm_Vertical -> Connector_PinHeader_2.54mm:PinHeader_2x07_P2.54mm_Vertical
- J11: value 3.3V_I2C -> Conn_01x04_Pin; footprint Connector_PinHeader_2.54mm:PinHeader_1x02_P2.54mm_Vertical -> Connector_PinHeader_2.54mm:PinHeader_1x04_P2.54mm_Vertical
- J2: value USB3_B -> Conn_01x03_Pin; footprint Connector_JST:JST_SH_BM09B-SRSS-TB_1x09-1MP_P1.00mm_Vertical -> Connector_PinHeader_2.00mm:PinHeader_1x03_P2.00mm_Vertical
- J4: value I2C_1 -> Conn_01x02_Pin; footprint Connector_PinHeader_2.54mm:PinHeader_1x02_P2.54mm_Vertical -> Connector_PinSocket_2.00mm:PinSocket_1x02_P2.00mm_Vertical
- J5: value I2C_2 -> Conn_01x02_Pin; footprint Connector_PinHeader_2.54mm:PinHeader_1x02_P2.54mm_Vertical -> Connector_PinSocket_2.00mm:PinSocket_1x02_P2.00mm_Vertical
- J6: value I2C_3 -> 3.3V_I2C
- J7: value I2C_4 -> Conn_01x10; footprint Connector_PinHeader_2.54mm:PinHeader_1x02_P2.54mm_Vertical -> Connector_PinHeader_2.54mm:PinHeader_1x10_P2.54mm_Vertical
- J8: value I2C_5 -> Conn_01x09_Pin; footprint Connector_PinHeader_2.54mm:PinHeader_1x02_P2.54mm_Vertical -> Connector_PinHeader_2.54mm:PinHeader_1x09_P2.54mm_Vertical
- J9: value I2C_6 -> Conn_Coaxial; footprint Connector_PinHeader_2.54mm:PinHeader_1x02_P2.54mm_Vertical -> Connector_Coaxial:SMA_Amphenol_132289_EdgeMount
- L2: value 1/2.2uH -> 2.2uH,5A
- L3: value 10uH 12A -> 1/2.2uH
- L5: value 2.2uH -> 10uH 12A
- L7: value 1uH -> 2.2uH
- L8: value 2.2uH,5A -> 1uH
- R1: value 10k -> 5.1kΩ
- R10: value 29.8k -> 10kΩ
- R102: value 10kΩ -> 249k
- R103: value 100kΩ -> 220Ω
- R104: value 124k -> 1kΩ
- R105: value 10k -> 1kΩ
- R106: value 549Ω -> 240Ω
- R107, R108: value 1kΩ -> 240Ω
- R11: value 120k -> 100k
- R110, R112, R122, R134: value 10kΩ -> 22Ω
- R116, R117, R123, R130: value 22Ω -> 10kΩ
- R12: value 10k -> 100k
- R124: value 22Ω -> 11kΩ
- R129: value 22Ω -> 470Ω
- R13: value 10k -> 100kΩ
- R132: value 10kΩ -> 470Ω
- R133: value 2.49kΩ -> 22Ω
- R135: value 2.49kΩ -> 5.1kΩ
- R136: value 11kΩ -> 22Ω
- R137: value 470Ω -> 8.06kΩ
- R138: value 470Ω -> 5.1kΩ
- R139: value 1kΩ -> 22Ω
- R14: value 10k -> 549Ω
- R140: value 8.06kΩ -> 1kΩ
- R142: value 5.1kΩ -> 2.49kΩ
- R143: value 5.1kΩ -> 10kΩ
- R144: value 47.5kΩ -> 2.49kΩ
- R145: value 22.1kΩ -> 1kΩ
- R146: value 1kΩ -> 47.5kΩ
- R147: value 2.2kΩ -> 22.1kΩ
- R148: value 2.2kΩ -> 1MΩ
- R149: value 10kΩ -> 2.2kΩ
- R15: value 10k -> 750Ω
- R151: value 2.2kΩ -> 10kΩ
- R153, R155: value 2.2kΩ -> 100kΩ
- R157: value 12kΩ -> 2.2kΩ
- R159: value 220Ω -> 2.2kΩ
- R16: value 100Ω -> 470R
- R160: value 5.1kΩ -> 2.2kΩ
- R161: value 5.1kΩ -> 12kΩ
- R162, R170, R80: value 100kΩ -> 10kΩ
- R163: value 100kΩ -> 5.1kΩ
- R164: value 1MΩ -> 5.1kΩ
- R165: value 1MΩ -> 100kΩ
- R169: value 100kΩ -> 33Ω
- R17: value 442k -> 470R
- R171: value 10kΩ -> 33Ω
- R18: value 10k -> 29.8k
- R19: value 10k -> 120k
- R2: value 22Ω -> 100kΩ
- R20: value 124k -> 10k
- R21: value 20.5k -> 10k
- R22: value 210k -> 10k
- R23, R29, R75: value 10kΩ -> 10k
- R24: value 180Ω -> 10k
- R25: value 5.23kΩ -> 124k
- R26: value 10kΩ -> 750Ω
- R28: value 10kΩ -> 5.9kΩ
- R3: value 240Ω -> 5.1kΩ
- R30: value 10kΩ -> 442k
- R31: value 10mΩ -> 210k; footprint Resistor_SMD:R_2512_6332Metric -> Resistor_SMD:R_0402_1005Metric
- R32: value 1kΩ -> 20.5k
- R33: value 30.1kΩ -> 10mΩ; footprint Resistor_SMD:R_0402_1005Metric -> Resistor_SMD:R_Shunt_Isabellenhuette_BVR4026
- R36, R51, R57, R79: value 100k -> 10kΩ
- R37, R48: value 10kΩ -> 1kΩ
- R38: value 10kΩ -> 1k
- R39: value 100kΩ -> 100
- R4: value 240Ω -> 10k
- R40: value 10kΩ -> 180Ω
- R41: value 73.2kΩ -> 100kΩ
- R42: value 249kΩ -> 30.1kΩ
- R44: value 309k -> 10kΩ
- R45: value 100k -> 5.23kΩ
- R46: value 50K -> 10kΩ
- R47: value 49.9k -> 10kΩ
- R49: value 24.3kΩ -> 100kΩ
- R5: value 240Ω -> 100Ω
- R50: value 60.4k -> 100kΩ
- R52: value 10Ω -> 100kΩ
- R53: value 200k -> 10kΩ
- R54, R56: value 100k -> 100kΩ
- R55: value 10k -> 31.6K
- R58: value 100k -> 60.4k
- R59: value 182kΩ -> 100kΩ
- R6, R8: value 470R -> 4.7kΩ
- R60: value 3.24kΩ -> 100k
- R61: value 14.7kΩ -> 10kΩ
- R62: value 49.9kΩ -> 10kΩ
- R63: value 49.9kΩ -> 49.9k
- R64: value 120k -> 24.3kΩ
- R65: value 20k -> 100k
- R67: value 249k -> 10Ω
- R69: value 10kΩ -> 73.2kΩ
- R7: value 750Ω -> 10k
- R70: value 249k -> 100k
- R71: value 10kΩ -> 249kΩ
- R72: value 20k -> 309k
- R73: value 50K -> 100k
- R76: value 4.7kΩ -> 100k
- R77: value 4.7kΩ -> 200k
- R81: value 1k -> 49.9kΩ
- R82: value 100 -> 49.9kΩ
- R85, R87: value 100kΩ -> 20k
- R86: value 100kΩ -> 50K
- R88: value 31.6K -> 182kΩ
- R89: value 10kΩ -> 50K
- R9: value 750Ω -> 124k
- R90: value 100kΩ -> 100k
- R91, R93: value 100kΩ -> 249k
- R92: value 5.9kΩ -> 120k
- R94: value 5.1kΩ -> 3.24kΩ
- R95: value 5.1kΩ -> 14.7kΩ
- R96: value 249k -> 10kΩ
- R98: value 1kΩ -> 10kΩ
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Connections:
- C1 pad 1: GND -> Net-(U2-VREG_1V2)
- C1 pad 2: VREG_2V7 -> GND
- C10 pad 1: Net-(U5-ITIMER) -> GND
- C10 pad 2: GND -> +3V3
- C100 pad 1: Net-(U25-SS/TRK) -> +5V_SYS
- C101 pad 1: +5V_SYS -> Net-(U22-NR)
- C102 pad 1: Net-(U25-COMP) -> Net-(U23-NR)
- C102 pad 2: Net-(C102-Pad2) -> GND
- C103 pad 1: Net-(C102-Pad2) -> GND
- C103 pad 2: GND -> PS_POR_B
- C104 pad 1: Net-(U25-FB) -> Net-(C104-Pad1)
- C104 pad 2: GND -> Net-(U25-BOOT)
- C105 pad 1: +0V9_GTR -> +5V_ANA
- C106 pad 2: +0V9_GTR -> +5V_ANA
- C107 pad 1: +1V2_GTH -> Net-(C107-Pad1)
- C108 pad 1: GND -> +5V_SYS
- C108 pad 2: +1V2_GTH -> GND
- C109 pad 1: +1V8_MGTRAVTT -> Net-(U25-SS/TRK)
- C11 pad 1: MUX_OUT -> GND
- C11 pad 2: GND -> Net-(U1-VBIAS)
- C110 pad 1: GND -> +5V_SYS
- C110 pad 2: +1V8_MGTRAVTT -> GND
- C111 pad 1: Net-(U24-DVDT) -> Net-(U25-COMP)
- C111 pad 2: GND -> Net-(C111-Pad2)
- C112 pad 1: +1V25 -> Net-(C111-Pad2)
- C113 pad 1: +1V2_PS -> +1V25
- C114 pad 1: GND -> Net-(U25-FB)
- C114 pad 2: +1V2_PS -> GND
- C115 pad 1: +1V8_VCCADC -> +0V9_VCU
- C116 pad 1: GND -> +0V9_VCU
- C116 pad 2: +1V8_VCCADC -> GND
- C117 pad 1: GND -> Net-(U26-NR)
- C117 pad 2: +0V85 -> GND
- C118 pad 1: GND -> +5V_SYS
- C118 pad 2: Net-(C118-Pad2) -> GND
- C119 pad 1: GND -> +0V9_GTR
- C119 pad 2: Net-(C119-Pad2) -> GND
- C12 pad 1: MUX_OUT -> Net-(U4-DVDT)
- C120 pad 2: Net-(C120-Pad2) -> +0V9_GTR
- C121 pad 2: Net-(C121-Pad2) -> +0V85
- C13 pad 1: +15V_MAIN -> GND
- C13 pad 2: GND -> PWR_CURR_MON_eF
- C131 pad 2: +0V85 -> Net-(C131-Pad2)
- C132 pad 2: +0V85 -> Net-(C132-Pad2)
- C133 pad 2: +0V85 -> Net-(C133-Pad2)
- C134 pad 2: +0V85 -> Net-(C134-Pad2)
- C136 pad 1: +0V85 -> GND
- C136 pad 2: GND -> +0V85
- C137 pad 1: Net-(C118-Pad2) -> GND
- C137 pad 2: GND -> +0V85
- C138 pad 1: Net-(C119-Pad2) -> GND
- C138 pad 2: GND -> +0V85
- C139 pad 1: Net-(C120-Pad2) -> GND
- C139 pad 2: GND -> +0V85
- C14 pad 1: U5_DVDT -> Net-(U5-SS)
- C140 pad 1: Net-(C121-Pad2) -> +0V85
- C15 pad 1: +15V_MAIN -> MUX_OUT
- C150 pad 1: +0V85 -> Net-(C131-Pad2)
- C151 pad 1: +0V85 -> Net-(C132-Pad2)
- C152 pad 1: +0V85 -> Net-(C133-Pad2)
- C153 pad 1: +0V85 -> Net-(C134-Pad2)
- C155 pad 1: GND -> +0V85
- C155 pad 2: +0V85_PS -> GND
- C156 pad 1: GND -> +0V85
- C156 pad 2: Net-(C156-Pad2) -> GND
- C157 pad 1: GND -> +0V85
- C157 pad 2: +0V85_PS -> GND
- C158 pad 1: GND -> +0V85
- C158 pad 2: +0V85_PS -> GND
- C159 pad 2: Net-(C159-Pad2) -> +0V85_PS
- C16 pad 1: Net-(U6-BTST) -> Net-(U6-ITIMER)
- C16 pad 2: Net-(C16-Pad2) -> GND
- C160 pad 2: +0V85_PS -> Net-(C160-Pad2)
- C162 pad 2: +0V9_VCU -> +0V85_PS
- C163 pad 2: +0V9_VCU -> Net-(C163-Pad2)
- C164 pad 2: +1V8 -> +0V85_PS
- C165 pad 2: +1V8 -> +0V85_PS
- C166 pad 2: +1V8 -> +0V9_VCU
- C167 pad 2: +1V8 -> +0V9_VCU
- C168 pad 2: +0V85_PS -> +1V8
- C169 pad 2: +0V85_PS -> +1V8
- C17 pad 1: /Battery.Charger,Fuel Gauge/REGN -> MUX_OUT
- C170 pad 1: +0V85_PS -> GND
- C170 pad 2: GND -> +1V8
- C172 pad 1: +0V85_PS -> GND
- C172 pad 2: GND -> +0V85_PS
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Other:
- board outline added: 174.2 x 169.9 mm
